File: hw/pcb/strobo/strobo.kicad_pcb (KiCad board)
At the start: 2 copper layers, 94.8 x 94.8 mm, 92 parts, among them J1 Conn_ARM_JTAG_SWD_10, SW1 SW_SPST, U1 ICM-20602, U2 STM32L051K8Ux, U3 Ring_Tracks, Y1 32kHz

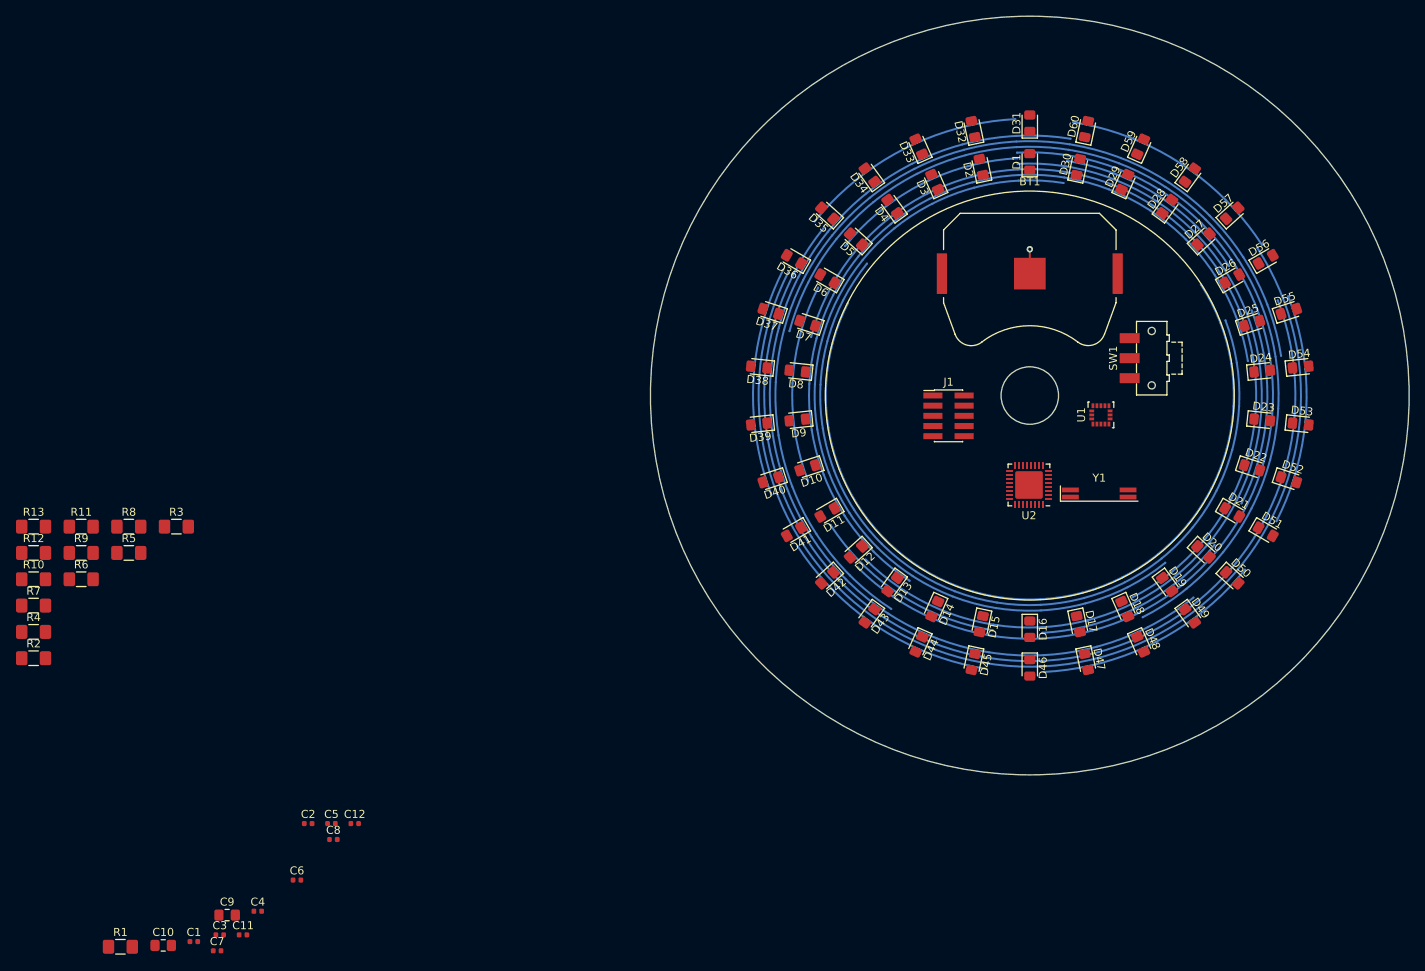
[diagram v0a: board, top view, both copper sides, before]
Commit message: major routing
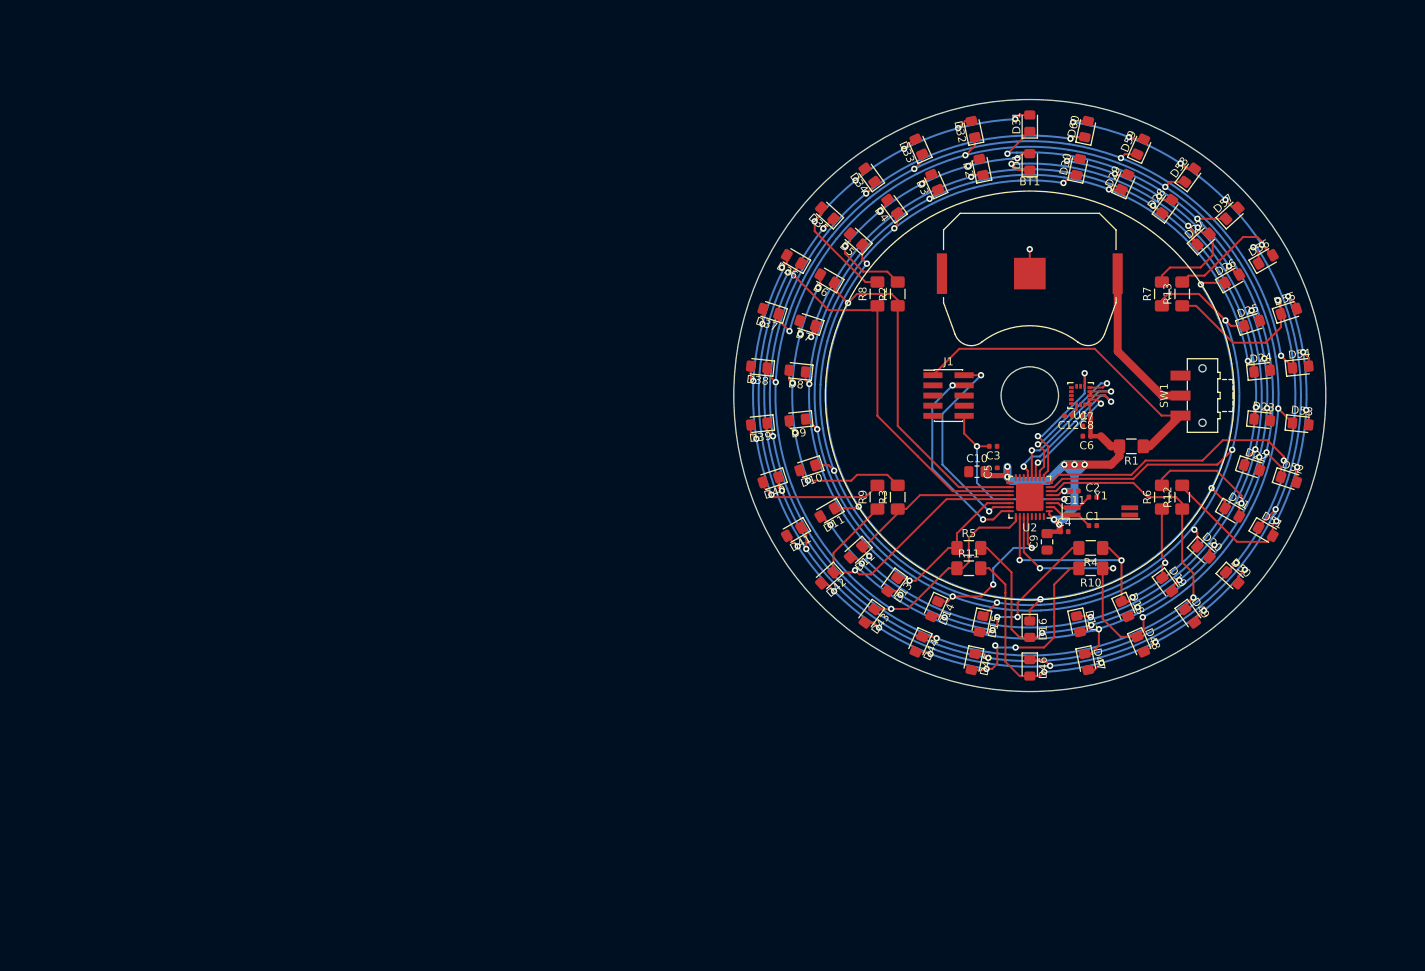
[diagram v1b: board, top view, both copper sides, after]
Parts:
- moved R13 146.5 mm to (219.7, 87.6), turned to 90 degrees
- moved R7 146.3 mm to (217.2, 87.6), turned to 90 degrees
- moved R12 143.7 mm to (219.7, 113.0), turned to 90 degrees
- moved R1 141.0 mm to (213.4, 106.7), turned to 180 degrees
- moved R6 135.5 mm to (217.2, 113.0), turned to 90 degrees
- moved R4 132.6 mm to (208.3, 119.4), turned to 180 degrees
- moved R10 132.2 mm to (208.3, 121.9), turned to 180 degrees
- moved C7 127.0 mm to (207.8, 104.1)
- moved C1 123.8 mm to (208.5, 116.6)
- moved C11 117.8 mm to (206.2, 112.3), turned to 180 degrees
- moved C10 117.7 mm to (194.1, 109.9)
- moved R2 117.2 mm to (184.2, 87.6), turned to 90 degrees
- moved C3 114.4 mm to (196.1, 106.7), turned to 180 degrees
- moved C6 113.2 mm to (207.8, 105.4), turned to 180 degrees
- moved C9 112.6 mm to (202.8, 118.6), turned to 90 degrees
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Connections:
- net /LED Matrix/LM_R_A renamed RA
- C6 pad 1: VDD -> Net-(C10-Pad2)
- C7 pad 2: VDD -> Net-(C10-Pad2)
- C8 pad 1: VDD -> Net-(C10-Pad2)
- D1 pad 1: /LED Matrix/LM_R_B -> RB
- D10 pad 1: /LED Matrix/LM_R_F -> RF
- D12 pad 1: /LED Matrix/LM_R_B -> RB
- D13 pad 1: /LED Matrix/LM_R_D -> RD
- D14 pad 1: /LED Matrix/LM_R_E -> RE
- D15 pad 1: /LED Matrix/LM_R_F -> RF
- D17 pad 1: /LED Matrix/LM_R_B -> RB
- D18 pad 1: /LED Matrix/LM_R_C -> RC
- D19 pad 1: /LED Matrix/LM_R_E -> RE
- D2 pad 1: /LED Matrix/LM_R_C -> RC
- D20 pad 1: /LED Matrix/LM_R_F -> RF
- D22 pad 1: /LED Matrix/LM_R_B -> RB
- D23 pad 1: /LED Matrix/LM_R_C -> RC
- D24 pad 1: /LED Matrix/LM_R_D -> RD
- D25 pad 1: /LED Matrix/LM_R_F -> RF
- D27 pad 1: /LED Matrix/LM_R_B -> RB
- D28 pad 1: /LED Matrix/LM_R_C -> RC
- D29 pad 1: /LED Matrix/LM_R_D -> RD
- D3 pad 1: /LED Matrix/LM_R_D -> RD
- D30 pad 1: /LED Matrix/LM_R_E -> RE
- D31 pad 1: /LED Matrix/LM_S_B -> SB
- D32 pad 1: /LED Matrix/LM_S_C -> SC
- D33 pad 1: /LED Matrix/LM_S_D -> SD
- D34 pad 1: /LED Matrix/LM_S_E -> SE
- D35 pad 1: /LED Matrix/LM_S_F -> SF
- D36 pad 1: /LED Matrix/LM_S_A -> SA
- D37 pad 1: /LED Matrix/LM_S_C -> SC
- D38 pad 1: /LED Matrix/LM_S_D -> SD
- D39 pad 1: /LED Matrix/LM_S_E -> SE
- D4 pad 1: /LED Matrix/LM_R_E -> RE
- D40 pad 1: /LED Matrix/LM_S_F -> SF
- D41 pad 1: /LED Matrix/LM_S_A -> SA
- D42 pad 1: /LED Matrix/LM_S_B -> SB
- D43 pad 1: /LED Matrix/LM_S_D -> SD
- D44 pad 1: /LED Matrix/LM_S_E -> SE
- D45 pad 1: /LED Matrix/LM_S_F -> SF
- D46 pad 1: /LED Matrix/LM_S_A -> SA
- D47 pad 1: /LED Matrix/LM_S_B -> SB
- D48 pad 1: /LED Matrix/LM_S_C -> SC
- D49 pad 1: /LED Matrix/LM_S_E -> SE
- D5 pad 1: /LED Matrix/LM_R_F -> RF
- D50 pad 1: /LED Matrix/LM_S_F -> SF
- D51 pad 1: /LED Matrix/LM_S_A -> SA
- D52 pad 1: /LED Matrix/LM_S_B -> SB
- D53 pad 1: /LED Matrix/LM_S_C -> SC
- D54 pad 1: /LED Matrix/LM_S_D -> SD
- D55 pad 1: /LED Matrix/LM_S_F -> SF
- D56 pad 1: /LED Matrix/LM_S_A -> SA
- D57 pad 1: /LED Matrix/LM_S_B -> SB
- D58 pad 1: /LED Matrix/LM_S_C -> SC
- D59 pad 1: /LED Matrix/LM_S_D -> SD
- D60 pad 1: /LED Matrix/LM_S_E -> SE
- D7 pad 1: /LED Matrix/LM_R_C -> RC
- D8 pad 1: /LED Matrix/LM_R_D -> RD
- D9 pad 1: /LED Matrix/LM_R_E -> RE
- R10 pad 1: /LED Matrix/LM_S_C -> SC
- R11 pad 1: /LED Matrix/LM_S_D -> SD
- R12 pad 1: /LED Matrix/LM_S_E -> SE
- R13 pad 1: /LED Matrix/LM_S_F -> SF
- R3 pad 1: /LED Matrix/LM_R_B -> RB
- R4 pad 1: /LED Matrix/LM_R_C -> RC
- R5 pad 1: /LED Matrix/LM_R_D -> RD
- R6 pad 1: /LED Matrix/LM_R_E -> RE
- R7 pad 1: /LED Matrix/LM_R_F -> RF
- R8 pad 1: /LED Matrix/LM_S_A -> SA
- R9 pad 1: /LED Matrix/LM_S_B -> SB
- U1 pad 1: VDD -> Net-(C10-Pad2)
- U1 pad 16: VDD -> Net-(C10-Pad2)
- U2 pad 19: /LED Matrix/LM_R_B -> SA
- U2 pad 20: /LED Matrix/LM_R_C -> RB
- U2 pad 21: /LED Matrix/LM_R_D -> SB
- U2 pad 22: /LED Matrix/LM_R_E -> RD
- U2 pad 25: /LED Matrix/LM_R_F -> SD
- U2 pad 26: /LED Matrix/LM_S_F -> RC
- U2 pad 27: /LED Matrix/LM_S_E -> SC
- U2 pad 28: /LED Matrix/LM_S_D -> RE
- U2 pad 29: /LED Matrix/LM_S_C -> Net-(U2-Pad29)
- U2 pad 30: /LED Matrix/LM_S_B -> Net-(U2-Pad30)
- U2 pad 32: /LED Matrix/LM_S_A -> Net-(U2-Pad32)
- U2 pad 6: Net-(U2-Pad6) -> SE
- U2 pad 7: Net-(U2-Pad7) -> RF
- U2 pad 8: Net-(U2-Pad8) -> SF
- U3 pad 10: /LED Matrix/LM_S_D -> SD
- U3 pad 11: /LED Matrix/LM_S_E -> SE
- U3 pad 12: /LED Matrix/LM_S_F -> SF
- U3 pad 13: /LED Matrix/LM_S_A -> SA
- U3 pad 2: /LED Matrix/LM_R_F -> RF
- U3 pad 3: /LED Matrix/LM_R_E -> RE
- U3 pad 4: /LED Matrix/LM_R_D -> RD
- U3 pad 5: /LED Matrix/LM_R_C -> RC
- U3 pad 6: /LED Matrix/LM_R_B -> RB
- U3 pad 8: /LED Matrix/LM_S_B -> SB
- U3 pad 9: /LED Matrix/LM_S_C -> SC
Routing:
- net SA: track 0.00 -> 64.9 mm, vias 0 -> 5
- net SF: track 0.00 -> 59.3 mm, vias 0 -> 6
- net Net-(C10-Pad2): track 0.00 -> 57.3 mm, vias 0 -> 8
- net SB: track 0.00 -> 56.4 mm, vias 0 -> 5
- net RA: track 0.00 -> 55.9 mm, vias 0 -> 5
- net RF: track 0.00 -> 48.1 mm, vias 0 -> 6
- net SC: track 0.00 -> 42.9 mm, vias 0 -> 7
- net VDD: track 0.00 -> 42.0 mm
- net SE: track 0.00 -> 39.9 mm, vias 0 -> 5
- net RB: track 0.00 -> 36.5 mm, vias 0 -> 5
- net RE: track 0.00 -> 34.8 mm, vias 0 -> 7
- net RC: track 0.00 -> 34.6 mm, vias 0 -> 7
- net SD: track 0.00 -> 33.4 mm, vias 0 -> 5
- net Net-(D41-Pad2): track 0.00 -> 32.4 mm, vias 0 -> 7
- net Net-(D46-Pad2): track 0.00 -> 27.4 mm, vias 0 -> 5
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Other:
- board size 94.8 x 94.8 mm -> 74 x 74 mm
